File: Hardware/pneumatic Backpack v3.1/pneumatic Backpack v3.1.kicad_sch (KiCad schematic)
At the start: 32 parts, among them J1 Conn_01x12_Pin, J10 Conn_01x02_Pin, J11 Conn_01x02_Pin, J2 Conn_01x01_Pin, J5 Conn_01x12_Pin, J9 Conn_01x02_Pin, U1 ESP32-S3-DEVKITC-1-N8R2, U5 MCZ33996EK

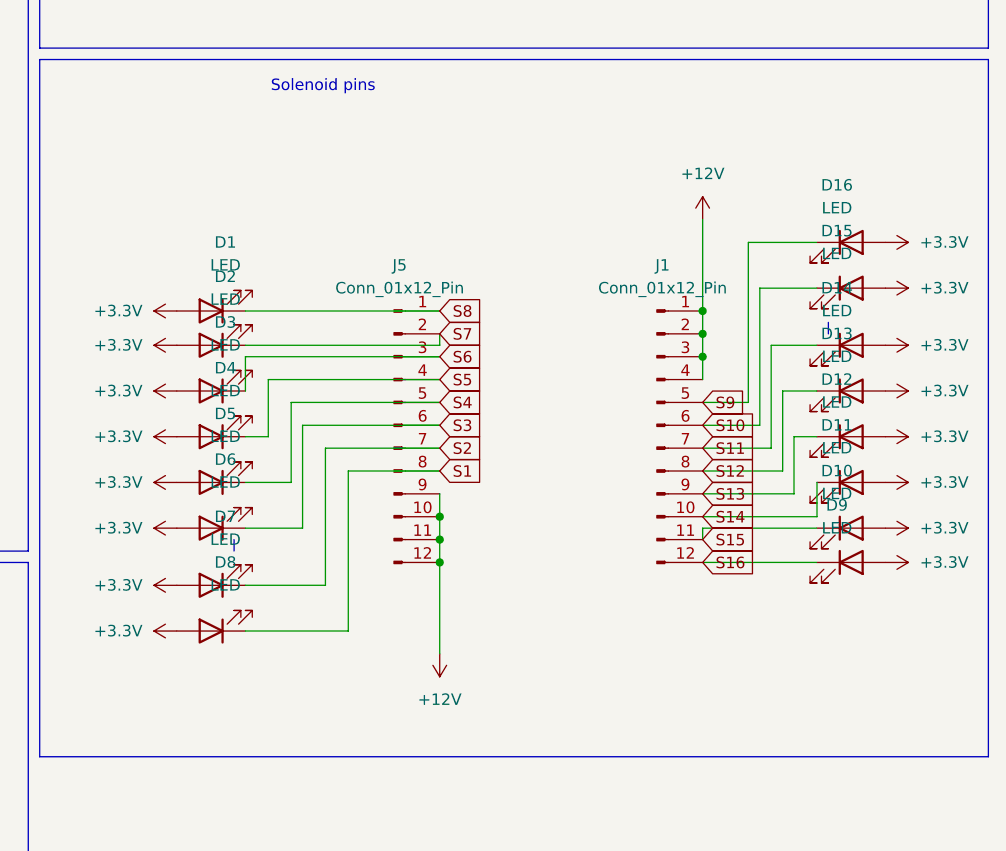
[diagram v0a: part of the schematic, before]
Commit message: updated
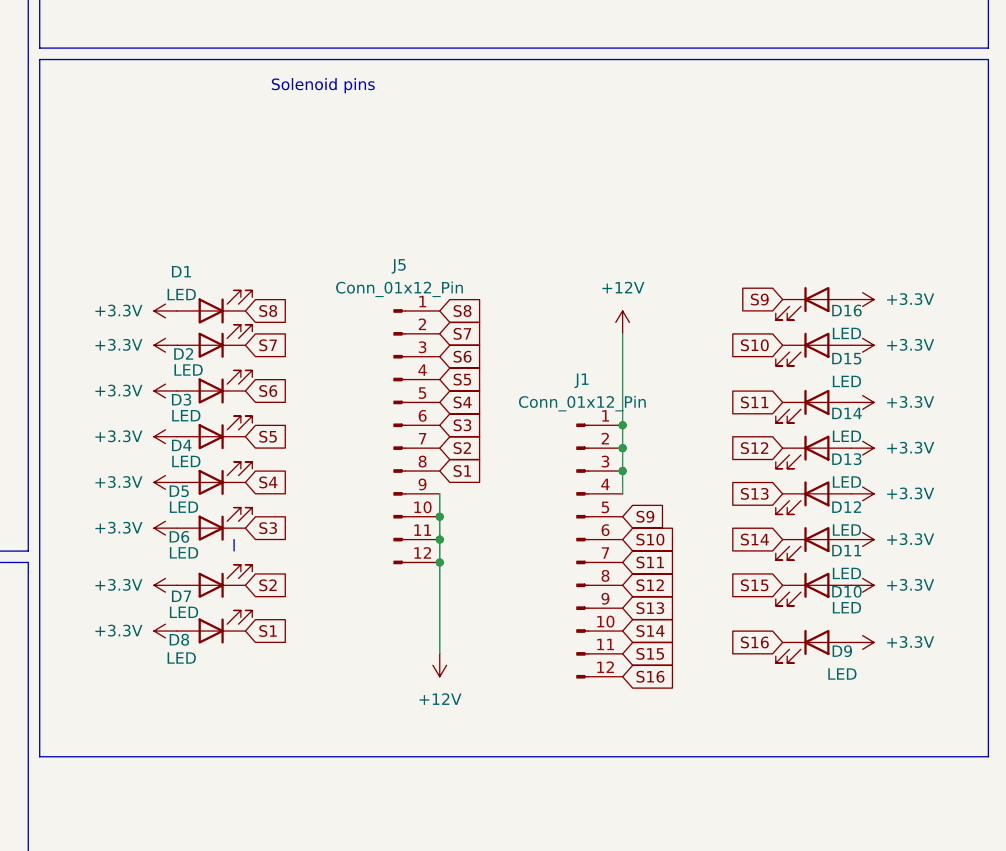
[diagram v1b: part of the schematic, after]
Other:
- moved on the sheet: D10, D11, D12, D13, D14, D15, D16, D9, J1
